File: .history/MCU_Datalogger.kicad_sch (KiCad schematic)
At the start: 25 parts, among them U1 24LC1025, U2 24LC1025, U3 DS1337S_, U4 ATMEGA328P-AU, Y1 32.768 KHz, Y2 16 MHz

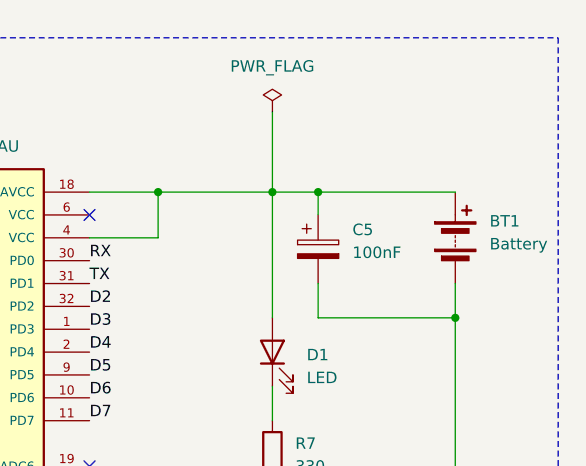
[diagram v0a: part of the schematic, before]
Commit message: all done board
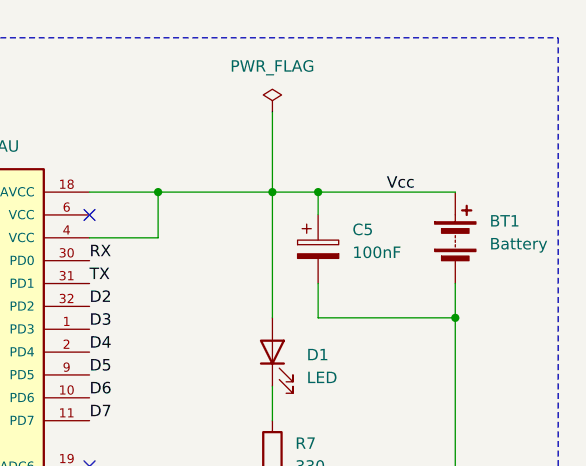
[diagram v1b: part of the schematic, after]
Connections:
- net Vcc: now also BT1.1 (+), C5.1, D1.2 (A), U4.18 (AVCC), U4.4 (VCC)
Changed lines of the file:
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@@
+		)
+	)
+	(label "Vcc"
+		(at 265.43 36.83 0)
+		(effects
+			(font
+				(size 1.27 1.27)
+			)
+			(justify left bottom)
 		)
 	)
